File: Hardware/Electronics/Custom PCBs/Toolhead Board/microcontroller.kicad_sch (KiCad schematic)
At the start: 35 parts, among them J1 USB C Receptacle, J2 Conn_02x08_Odd_Even, J3 Conn_02x08_Odd_Even, J4 Conn_02x08_Odd_Even, J5 Conn_02x04_Odd_Even, J6 Conn_02x04_Odd_Even, SW1 BOOT, SW2 RESET, U3 RP2040, U4 W25Q128JVS, Y1 12MHz/12pF/50Ω/20ppm

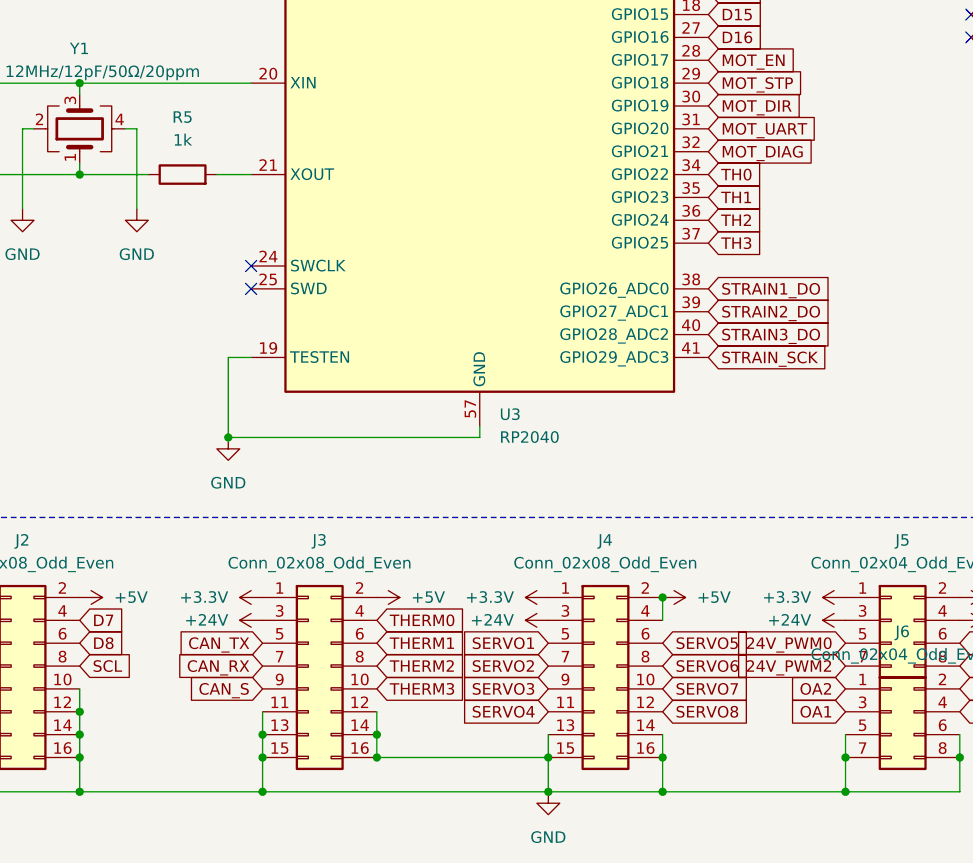
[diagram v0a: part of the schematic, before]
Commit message: Update layout
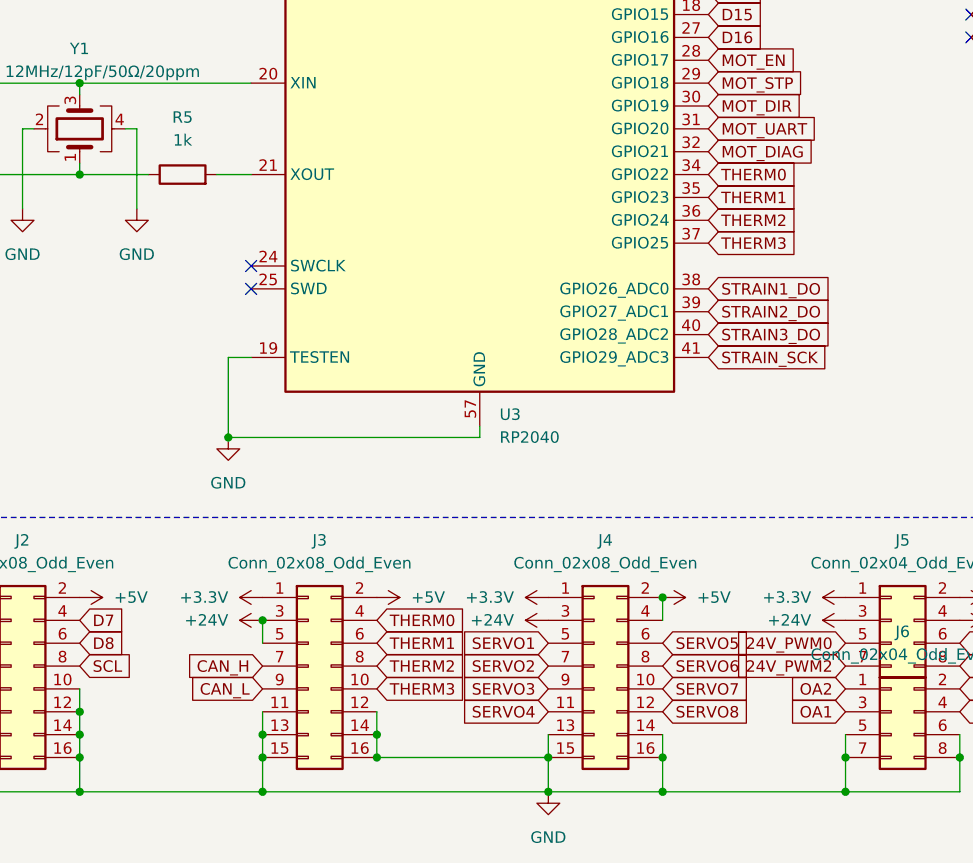
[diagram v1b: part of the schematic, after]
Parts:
- J1: footprint Connector_USB:USB_C_Receptacle_GCT_USB4105-xx-A_16P_TopMnt_Horizontal -> Connector_USB:USB_C_Receptacle_JAE_DX07S016JA1R1500
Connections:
- net TH0 is gone; now on net THERM0: U3.34 (GPIO22)
- net TH1 is gone; now on net THERM1: U3.35 (GPIO23)
- net TH2 is gone; now on net THERM2: U3.36 (GPIO24)
- net TH3 is gone; now on net THERM3: U3.37 (GPIO25)
- net +24V: now also J3.5 (Pin_5)
- net CAN_RX: no longer J3.7 (Pin_7)
- net CAN_S: no longer J3.9 (Pin_9)
- net CAN_TX: no longer J3.5 (Pin_5)
- new net CAN_H: J3.7 (Pin_7)
- new net CAN_L: J3.9 (Pin_9)
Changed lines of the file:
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@@
 	)
 	(junction
+		(at 59.69 147.32)
+		(diameter 0)
+		(color 0 0 0 0)
+	)
+	(junction
 		(at 104.14 162.56)
 		(diameter 0)
@@
 	(wire
 		(pts
+			(xy 59.69 147.32) (xy 59.69 149.86)
+		)
+		(stroke
+			(width 0)
+			(type default)
+		)
+	)
+	(wire
+		(pts
 			(xy 93.98 31.75) (xy 96.52 31.75)
 		)
@@
 		)
 	)
+	(global_label "THERM0"
+		(shape input)
+		(at 109.22 97.79 0)
+		(fields_autoplaced yes)
+		(effects
+			(font
+				(size 1.27 1.27)
+			)
+			(justify left)
+		)
+		(property "Intersheetrefs" "${INTERSHEET_REFS}"
+			(at 119.5832 97.79 0)
+			(effects
+				(font
+					(size 1.27 1.27)
+				)
+				(justify left)
+				(hide yes)
+			)
+		)
+	)
 	(global_label "24V_PWM2"
 		(shape input)
@@
 		)
 	)
-	(global_label "TH3"
-		(shape input)
-		(at 109.22 105.41 0)
-		(fields_autoplaced yes)
-		(effects
-			(font
-				(size 1.27 1.27)
-			)
-			(justify left)
-		)
-		(property "Intersheetrefs" "${INTERSHEET_REFS}"
-			(at 115.7128 105.41 0)
-			(effects
-				(font
-					(size 1.27 1.27)
-				)
-				(justify left)
-				(hide yes)
-			)
-		)
-	)
 	(global_label "OA1"
 		(shape input)
@@
 		)
 	)
-	(global_label "CAN_S"
-		(shape input)
-		(at 59.69 154.94 180)
-		(fields_autoplaced yes)
-		(effects
-			(font
-				(size 1.27 1.27)
-			)
-			(justify right)
-		)
-		(property "Intersheetrefs" "${INTERSHEET_REFS}"
-			(at 50.8386 154.94 0)
-			(effects
-				(font
-					(size 1.27 1.27)
-				)
-				(justify right)
-				(hide yes)
-			)
-		)
-	)
 	(global_label "OA2"
 		(shape input)
@@
 		)
 	)
-	(global_label "TH0"
-		(shape input)
-		(at 109.22 97.79 0)
-		(fields_autoplaced yes)
-		(effects
-			(font
-				(size 1.27 1.27)
-			)
-			(justify left)
-		)
-		(property "Intersheetrefs" "${INTERSHEET_REFS}"
-			(at 115.7128 97.79 0)
-			(effects
-				(font
-					(size 1.27 1.27)
-				)
-				(justify left)
-				(hide yes)
-			)
-		)
-	)
 	(global_label "MOT_UART"
 		(shape input)
@@
 		)
 	)
-	(global_label "CAN_TX"
-		(shape input)
-		(at 59.69 149.86 180)
-		(fields_autoplaced yes)
-		(effects
-			(font
-				(size 1.27 1.27)
-			)
-			(justify right)
-		)
-		(property "Intersheetrefs" "${INTERSHEET_REFS}"
-			(at 49.871 149.86 0)
-			(effects
-				(font
-					(size 1.27 1.27)
-				)
-				(justify right)
-				(hide yes)
-			)
-		)
-	)
 	(global_label "SDA"
 		(shape input)
@@
 		)
 	)
-	(global_label "TH1"
+	(global_label "THERM3"
 		(shape input)
-		(at 109.22 100.33 0)
+		(at 109.22 105.41 0)
 		(fields_autoplaced yes)
 		(effects
@@
 		)
 		(property "Intersheetrefs" "${INTERSHEET_REFS}"
-			(at 115.7128 100.33 0)
+			(at 119.5832 105.41 0)
 			(effects
 				(font
@@
 		)
 	)
+	(global_label "CAN_L"
+		(shape input)
+		(at 59.69 154.94 180)
+		(fields_autoplaced yes)
+		(effects
+			(font
+				(size 1.27 1.27)
+			)
+			(justify right)
+		)
+		(property "Intersheetrefs" "${INTERSHEET_REFS}"
+			(at 51.02 154.94 0)
+			(effects
+				(font
+					(size 1.27 1.27)
+				)
+				(justify right)
+				(hide yes)
+			)
+		)
+	)
+	(global_label "THERM1"
+		(shape input)
+		(at 109.22 100.33 0)
+		(fields_autoplaced yes)
+		(effects
+			(font
+				(size 1.27 1.27)
+			)
+			(justify left)
+		)
+		(property "Intersheetrefs" "${INTERSHEET_REFS}"
+			(at 119.5832 100.33 0)
+			(effects
+				(font
+					(size 1.27 1.27)
+				)
+				(justify left)
+				(hide yes)
+			)
+		)
+	)
 	(global_label "SERVO6"
 		(shape input)
@@
 		)
 	)
-	(global_label "CAN_RX"
+	(global_label "SERVO3"
 		(shape input)
-		(at 59.69 152.4 180)
+		(at 91.44 154.94 180)
 		(fields_autoplaced yes)
 		(effects
@@
 		)
 		(property "Intersheetrefs" "${INTERSHEET_REFS}"
-			(at 49.5686 152.4 0)
+			(at 81.1977 154.94 0)
 			(effects
 				(font
@@
 		)
 	)
-	(global_label "SERVO3"
+	(global_label "D0"
 		(shape input)
-		(at 91.44 154.94 180)
+		(at 109.22 41.91 0)
 		(fields_autoplaced yes)
 		(effects
@@
 				(size 1.27 1.27)
 			)
-			(justify right)
+			(justify left)
 		)
 		(property "Intersheetrefs" "${INTERSHEET_REFS}"
-			(at 81.1977 154.94 0)
+			(at 114.6847 41.91 0)
 			(effects
 				(font
 					(size 1.27 1.27)
 				)
-				(justify right)
+				(justify left)
 				(hide yes)
 			)
 		)
 	)
-	(global_label "D0"
+	(global_label "D11"
 		(shape input)
-		(at 109.22 41.91 0)
+		(at 109.22 69.85 0)
 		(fields_autoplaced yes)
 		(effects
@@
 		)
 		(property "Intersheetrefs" "${INTERSHEET_REFS}"
-			(at 114.6847 41.91 0)
+			(at 115.8942 69.85 0)
 			(effects
 				(font
@@
 		)
 	)
-	(global_label "TH2"
+	(global_label "MOT_STP"
 		(shape input)
-		(at 109.22 102.87 0)
+		(at 109.22 87.63 0)
 		(fields_autoplaced yes)
 		(effects
@@
 		)
 		(property "Intersheetrefs" "${INTERSHEET_REFS}"
-			(at 115.7128 102.87 0)
+			(at 120.3694 87.63 0)
 			(effects
 				(font
@@
 		)
 	)
-	(global_label "D11"
+	(global_label "CAN_H"
 		(shape input)
-		(at 109.22 69.85 0)
+		(at 59.69 152.4 180)
 		(fields_autoplaced yes)
 		(effects
@@
 				(size 1.27 1.27)
 			)
-			(justify left)
+			(justify right)
 		)
 		(property "Intersheetrefs" "${INTERSHEET_REFS}"
-			(at 115.8942 69.85 0)
+			(at 50.7176 152.4 0)
 			(effects
 				(font
 					(size 1.27 1.27)
 				)
-				(justify left)
+				(justify right)
 				(hide yes)
 			)
 		)
 	)
-	(global_label "MOT_STP"
+	(global_label "THERM2"
 		(shape input)
-		(at 109.22 87.63 0)
+		(at 109.22 102.87 0)
 		(fields_autoplaced yes)
 		(effects
@@
 		)
 		(property "Intersheetrefs" "${INTERSHEET_REFS}"
-			(at 120.3694 87.63 0)
+			(at 119.5832 102.87 0)
 			(effects
 				(font
@@
 			)
 		)
-		(property "Footprint" "Connector_USB:USB_C_Receptacle_GCT_USB4105-xx-A_16P_TopMnt_Horizontal"
+		(property "Footprint" "Connector_USB:USB_C_Receptacle_JAE_DX07S016JA1R1500"
 			(at 208.28 134.62 0)
 			(effects
